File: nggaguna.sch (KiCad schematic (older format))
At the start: 89 parts, among them U1 promicro

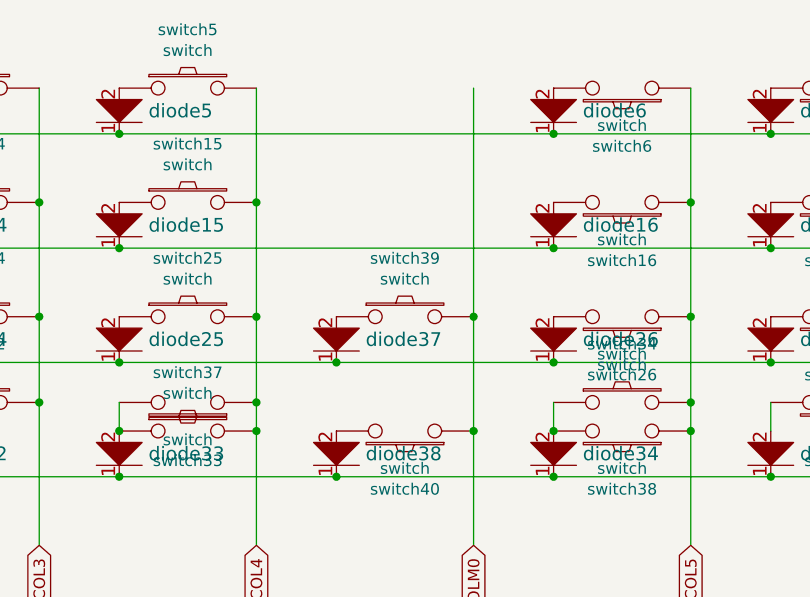
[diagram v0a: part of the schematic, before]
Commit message: revamp
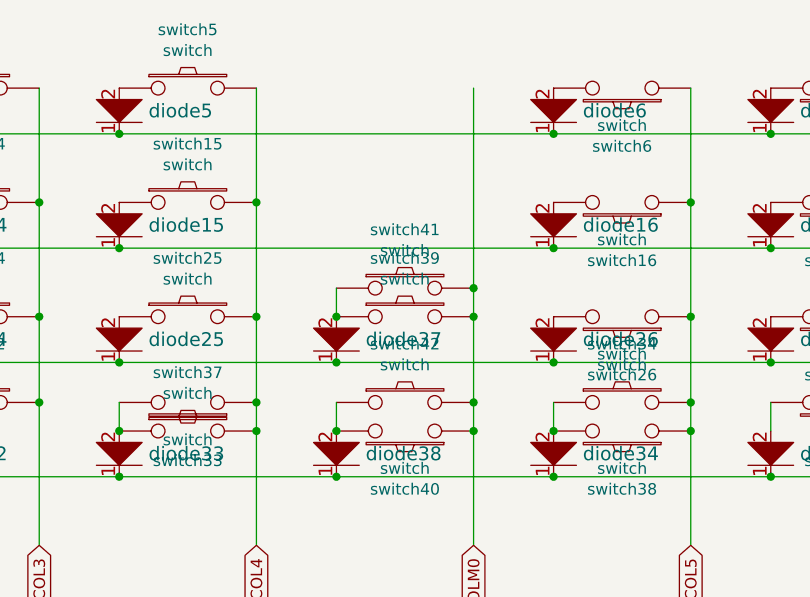
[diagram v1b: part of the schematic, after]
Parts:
- added switch41, switch42: switch, footprints:200-minimal, symbol rick:switch
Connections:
- net COLM0: now also switch41.2, switch42.2
- net at diode37.2, switch39.1: now also switch41.1
- net at diode38.2, switch40.2: now also switch42.1
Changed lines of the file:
@@
 Connection ~ 7600 2500
-$Comp
-L rick:switch switch39
-U 1 1 602125DC
-P 6000 1800
-F 0 "switch39" H 6000 2055 50  0000 C CNN
-F 1 "switch" H 6000 1964 50  0000 C CNN
-F 2 "footprints:100-minimal" H 6000 1800 60  0001 C CNN
-F 3 "" H 6000 1800 60  0000 C CNN
-	1    6000 1800
-	1    0    0    -1
-$EndComp
 $Comp
 L rick:diode diode37
@@
 Wire Wire Line
 	5700 2000 6650 2000
-Connection ~ 6300 1800
-Wire Wire Line
-	6300 1800 6300 2300
 Wire Wire Line
 	4750 1000 6650 1000
@@
 Wire Wire Line
 	4750 1500 6650 1500
-Wire Wire Line
-	6300 800  6300 1800
 Wire Wire Line
 	5350 1800 5350 2175
@@
 	1    0    0    -1
 $EndComp
+Wire Wire Line
+	6300 1800 6300 2175
+Connection ~ 6300 1800
+Wire Wire Line
+	6300 800  6300 1675
+$Comp
+L rick:switch switch39
+U 1 1 602125DC
+P 6000 1800
+F 0 "switch39" H 6000 2055 50  0000 C CNN
+F 1 "switch" H 6000 1964 50  0000 C CNN
+F 2 "footprints:100-minimal" H 6000 1800 60  0001 C CNN
+F 3 "" H 6000 1800 60  0000 C CNN
+	1    6000 1800
+	1    0    0    -1
+$EndComp
+$Comp
+L rick:switch switch41
+U 1 1 60293267
+P 6000 1675
+F 0 "switch41" H 6000 1930 50  0000 C CNN
+F 1 "switch" H 6000 1839 50  0000 C CNN
+F 2 "footprints:200-minimal" H 6000 1675 60  0001 C CNN
+F 3 "" H 6000 1675 60  0000 C CNN
+	1    6000 1675
+	1    0    0    -1
+$EndComp
+Connection ~ 6300 1675
+Wire Wire Line
+	6300 1675 6300 1800
+$Comp
+L rick:switch switch42
+U 1 1 60293F2B
+P 6000 2175
+F 0 "switch42" H 6000 2430 50  0000 C CNN
+F 1 "switch" H 6000 2339 50  0000 C CNN
+F 2 "footprints:200-minimal" H 6000 2175 60  0001 C CNN
+F 3 "" H 6000 2175 60  0000 C CNN
+	1    6000 2175
+	1    0    0    -1
+$EndComp
+Connection ~ 6300 2175
+Wire Wire Line
+	6300 2175 6300 2300
+Wire Wire Line
+	5700 2175 5700 2300
+Connection ~ 5700 2300
+Wire Wire Line
+	5700 1675 5700 1800
+Connection ~ 5700 1800
 $EndSCHEMATC
